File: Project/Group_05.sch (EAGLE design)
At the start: 29 parts, among them J1 POWER_JACKPTH_LOCK, U1 +12v, U3 TCA9546A_SMD

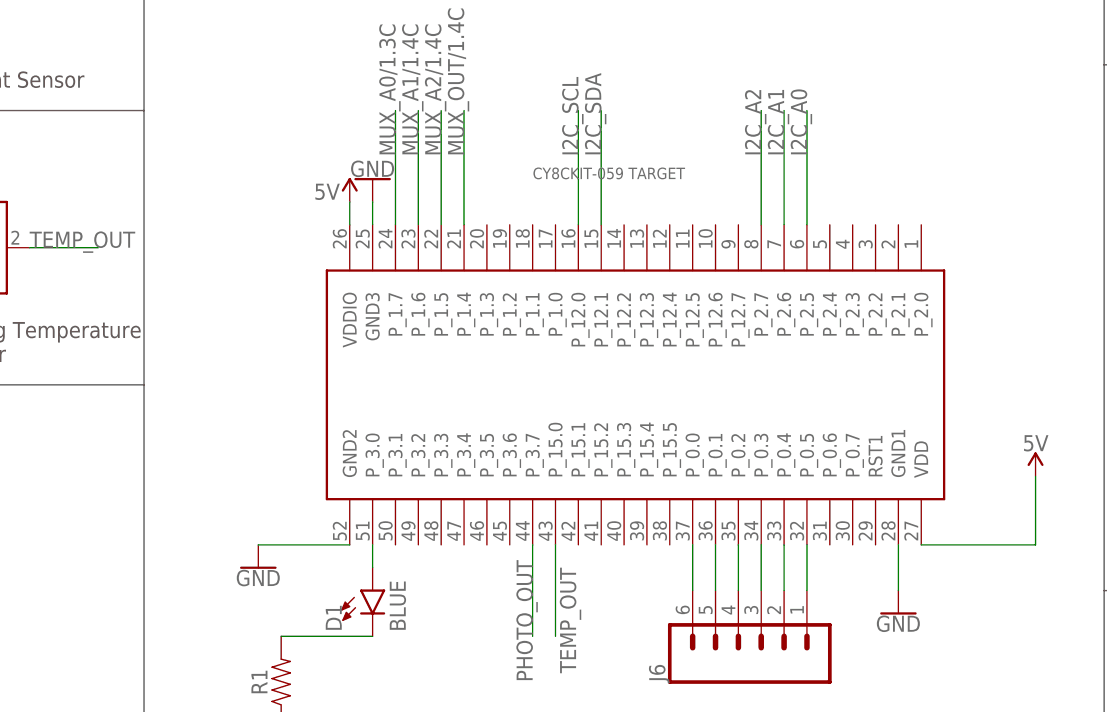
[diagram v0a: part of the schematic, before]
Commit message: brd placement
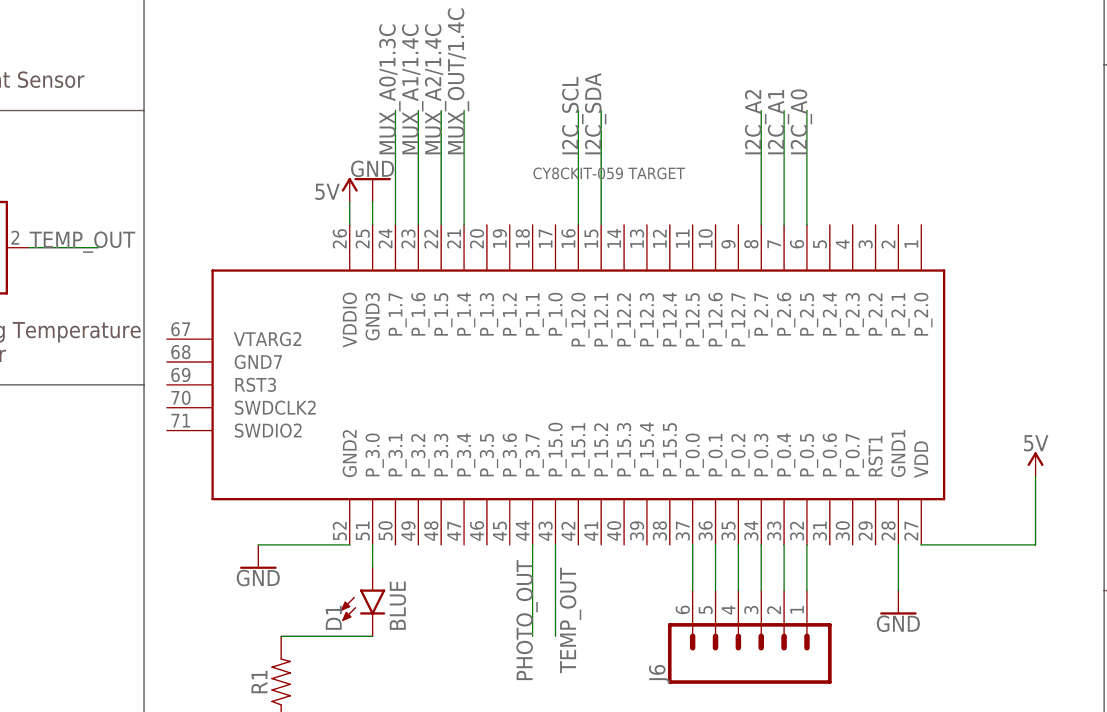
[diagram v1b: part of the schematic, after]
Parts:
- removed U$3: CY8CKIT-059_TARGET_3, CY8KIT-059:CY8CKIT-059_TARGET_3
- added U$1: CY8CKIT-059_TARGET, CY8KIT-059:CY8CKIT-059_TARGET
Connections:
- net 5V: now also U$1.VDD, U$1.VDDIO; no longer U$3.VDD, U$3.VDDIO
- net GND: now also U$1.GND1, U$1.GND2, U$1.GND3; no longer U$3.GND1, U$3.GND2, U$3.GND3
- net I2C_A0: now also U$1.P_2.5; no longer U$3.P_2.5
- net I2C_A1: now also U$1.P_2.6; no longer U$3.P_2.6
- net I2C_A2: now also U$1.P_2.7; no longer U$3.P_2.7
- net I2C_SCL: now also U$1.P_12.0; no longer U$3.P_12.0
- net I2C_SDA: now also U$1.P_12.1; no longer U$3.P_12.1
- net MUX_A0/1.3C: now also U$1.P_1.7; no longer U$3.P_1.7
- net MUX_A1/1.4C: now also U$1.P_1.6; no longer U$3.P_1.6
- net MUX_A2/1.4C: now also U$1.P_1.5; no longer U$3.P_1.5
- net MUX_OUT/1.4C: now also U$1.P_1.4; no longer U$3.P_1.4
- net N$1: now also U$1.P_0.0; no longer U$3.P_0.0
- net N$2: now also U$1.P_3.0; no longer U$3.P_3.0
- net N$5: now also U$1.P_0.1; no longer U$3.P_0.1
- net N$6: now also U$1.P_0.2; no longer U$3.P_0.2
- net N$7: now also U$1.P_0.3; no longer U$3.P_0.3
- net N$8: now also U$1.P_0.4; no longer U$3.P_0.4
- net N$9: now also U$1.P_0.5; no longer U$3.P_0.5
- net PHOTO_OUT: now also U$1.P_3.7; no longer U$3.P_3.7
- net TEMP_OUT: now also U$1.P_15.0; no longer U$3.P_15.0
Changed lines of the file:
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@@
 <part name="SUPPLY11" library="SparkFun-PowerSymbols" deviceset="5V" device=""/>
 <part name="U$2" library="Group_05_Library" deviceset="TMUX1208" device="_SMD"/>
-<part name="U$3" library="CY8KIT-059" deviceset="CY8CKIT-059_TARGET_3" device=""/>
 <part name="J8" library="SparkFun-Connectors" deviceset="CONN_08" device="LOCK"/>
 <part name="GND4" library="SparkFun-PowerSymbols" deviceset="GND" device=""/>
 <part name="GND5" library="SparkFun-PowerSymbols" deviceset="GND" device=""/>
 <part name="SUPPLY9" library="SparkFun-PowerSymbols" deviceset="5V" device=""/>
+<part name="U$1" library="CY8KIT-059" deviceset="CY8CKIT-059_TARGET" device=""/>
 </parts>
 <sheets>
@@
 <attribute name="VALUE" x="218.44" y="50.8" size="2.54" layer="96"/>
 </instance>
-<instance part="U$3" gate="G$1" x="93.98" y="71.12" smashed="yes"/>
 <instance part="J8" gate="G$1" x="187.96" y="55.88" smashed="yes">
 <attribute name="VALUE" x="182.88" y="43.434" size="1.778" layer="96" font="vector"/>
@@
 <attribute name="VALUE" x="60.96" y="91.694" size="1.778" layer="96" align="bottom-center"/>
 </instance>
+<instance part="U$1" gate="G$1" x="40.64" y="71.12" smashed="yes"/>
 </instances>
 <busses>
@@
 <pinref part="GND8" gate="1" pin="GND"/>
 <wire x1="124.46" y1="53.34" x2="124.46" y2="48.26" width="0.1524" layer="91"/>
-<pinref part="U$3" gate="G$1" pin="GND1"/>
+<pinref part="U$1" gate="G$1" pin="GND1"/>
 </segment>
 <segment>
@@
 <segment>
 <pinref part="GND4" gate="1" pin="GND"/>
-<pinref part="U$3" gate="G$1" pin="GND2"/>
 <wire x1="53.34" y1="53.34" x2="63.5" y2="53.34" width="0.1524" layer="91"/>
+<pinref part="U$1" gate="G$1" pin="GND2"/>
 </segment>
 <segment>
 <pinref part="GND5" gate="1" pin="GND"/>
-<pinref part="U$3" gate="G$1" pin="GND3"/>
 <wire x1="66.04" y1="91.44" x2="66.04" y2="88.9" width="0.1524" layer="91"/>
+<pinref part="U$1" gate="G$1" pin="GND3"/>
 </segment>
 </net>
@@
 <wire x1="139.7" y1="53.34" x2="139.7" y2="60.96" width="0.1524" layer="91"/>
 <pinref part="SUPPLY8" gate="G$1" pin="5V"/>
-<pinref part="U$3" gate="G$1" pin="VDD"/>
+<pinref part="U$1" gate="G$1" pin="VDD"/>
 </segment>
 <segment>
@@
 <segment>
 <pinref part="SUPPLY9" gate="G$1" pin="5V"/>
-<pinref part="U$3" gate="G$1" pin="VDDIO"/>
+<pinref part="U$1" gate="G$1" pin="VDDIO"/>
 <wire x1="63.5" y1="91.44" x2="63.5" y2="88.9" width="0.1524" layer="91"/>
 </segment>
@@
 <wire x1="83.82" y1="53.34" x2="83.82" y2="43.18" width="0.1524" layer="91"/>
 <label x="83.82" y="38.1" size="1.778" layer="95" rot="R90"/>
-<pinref part="U$3" gate="G$1" pin="P_3.7"/>
+<pinref part="U$1" gate="G$1" pin="P_3.7"/>
 </segment>
 </net>
@@
 <wire x1="86.36" y1="53.34" x2="86.36" y2="43.18" width="0.1524" layer="91"/>
 <label x="86.868" y="50.8" size="1.778" layer="95" rot="R270"/>
-<pinref part="U$3" gate="G$1" pin="P_15.0"/>
+<pinref part="U$1" gate="G$1" pin="P_15.0"/>
 </segment>
 </net>
@@
 <wire x1="91.44" y1="88.9" x2="91.44" y2="101.6" width="0.1524" layer="91"/>
 <label x="91.44" y="96.52" size="1.778" layer="95" rot="R90"/>
-<pinref part="U$3" gate="G$1" pin="P_12.1"/>
+<pinref part="U$1" gate="G$1" pin="P_12.1"/>
 </segment>
 </net>
@@
 <wire x1="88.9" y1="88.9" x2="88.9" y2="101.6" width="0.1524" layer="91"/>
 <label x="88.9" y="96.52" size="1.778" layer="95" rot="R90"/>
-<pinref part="U$3" gate="G$1" pin="P_12.0"/>
+<pinref part="U$1" gate="G$1" pin="P_12.0"/>
 </segment>
 </net>
@@
 <wire x1="114.3" y1="88.9" x2="114.3" y2="101.6" width="0.1524" layer="91"/>
 <label x="114.3" y="96.52" size="1.778" layer="95" rot="R90"/>
-<pinref part="U$3" gate="G$1" pin="P_2.5"/>
+<pinref part="U$1" gate="G$1" pin="P_2.5"/>
 </segment>
 </net>
@@
 <wire x1="111.76" y1="88.9" x2="111.76" y2="101.6" width="0.1524" layer="91"/>
 <label x="111.76" y="96.52" size="1.778" layer="95" rot="R90"/>
-<pinref part="U$3" gate="G$1" pin="P_2.6"/>
+<pinref part="U$1" gate="G$1" pin="P_2.6"/>
 </segment>
 </net>
@@
 <wire x1="109.22" y1="88.9" x2="109.22" y2="101.6" width="0.1524" layer="91"/>
 <label x="109.22" y="96.52" size="1.778" layer="95" rot="R90"/>
-<pinref part="U$3" gate="G$1" pin="P_2.7"/>
+<pinref part="U$1" gate="G$1" pin="P_2.7"/>
 </segment>
 </net>
@@
 <pinref part="D1" gate="G$1" pin="A"/>
 <wire x1="66.04" y1="53.34" x2="66.04" y2="50.8" width="0.1524" layer="91"/>
-<pinref part="U$3" gate="G$1" pin="P_3.0"/>
+<pinref part="U$1" gate="G$1" pin="P_3.0"/>
 </segment>
 </net>
@@
 <pinref part="J6" gate="G$1" pin="6"/>
 <wire x1="101.6" y1="53.34" x2="101.6" y2="48.26" width="0.1524" layer="91"/>
-<pinref part="U$3" gate="G$1" pin="P_0.0"/>
+<pinref part="U$1" gate="G$1" pin="P_0.0"/>
 </segment>
 </net>
@@
 <pinref part="J6" gate="G$1" pin="5"/>
 <wire x1="104.14" y1="53.34" x2="104.14" y2="48.26" width="0.1524" layer="91"/>
-<pinref part="U$3" gate="G$1" pin="P_0.1"/>
+<pinref part="U$1" gate="G$1" pin="P_0.1"/>
 </segment>
 </net>
@@
 <pinref part="J6" gate="G$1" pin="4"/>
 <wire x1="106.68" y1="53.34" x2="106.68" y2="48.26" width="0.1524" layer="91"/>
-<pinref part="U$3" gate="G$1" pin="P_0.2"/>
+<pinref part="U$1" gate="G$1" pin="P_0.2"/>
 </segment>
 </net>
@@
 <pinref part="J6" gate="G$1" pin="3"/>
 <wire x1="109.22" y1="53.34" x2="109.22" y2="48.26" width="0.1524" layer="91"/>
-<pinref part="U$3" gate="G$1" pin="P_0.3"/>
+<pinref part="U$1" gate="G$1" pin="P_0.3"/>
 </segment>
 </net>
@@
 <pinref part="J6" gate="G$1" pin="2"/>
 <wire x1="111.76" y1="53.34" x2="111.76" y2="48.26" width="0.1524" layer="91"/>
-<pinref part="U$3" gate="G$1" pin="P_0.4"/>
+<pinref part="U$1" gate="G$1" pin="P_0.4"/>
 </segment>
 </net>
@@
 <pinref part="J6" gate="G$1" pin="1"/>
 <wire x1="114.3" y1="53.34" x2="114.3" y2="48.26" width="0.1524" layer="91"/>
-<pinref part="U$3" gate="G$1" pin="P_0.5"/>
+<pinref part="U$1" gate="G$1" pin="P_0.5"/>
 </segment>
 </net>
@@
 <wire x1="68.58" y1="88.9" x2="68.58" y2="101.6" width="0.1524" layer="91"/>
 <label x="68.58" y="96.52" size="1.778" layer="95" rot="R90"/>
-<pinref part="U$3" gate="G$1" pin="P_1.7"/>
+<pinref part="U$1" gate="G$1" pin="P_1.7"/>
 </segment>
 </net>
@@
 <wire x1="71.12" y1="88.9" x2="71.12" y2="101.6" width="0.1524" layer="91"/>
 <label x="71.12" y="96.52" size="1.778" layer="95" rot="R90"/>
-<pinref part="U$3" gate="G$1" pin="P_1.6"/>
+<pinref part="U$1" gate="G$1" pin="P_1.6"/>
 </segment>
 </net>
@@
 <wire x1="73.66" y1="88.9" x2="73.66" y2="101.6" width="0.1524" layer="91"/>
 <label x="73.66" y="96.52" size="1.778" layer="95" rot="R90"/>
-<pinref part="U$3" gate="G$1" pin="P_1.5"/>
+<pinref part="U$1" gate="G$1" pin="P_1.5"/>
 </segment>
 </net>
@@
 <wire x1="76.2" y1="88.9" x2="76.2" y2="101.6" width="0.1524" layer="91"/>
 <label x="76.2" y="96.52" size="1.778" layer="95" rot="R90"/>
-<pinref part="U$3" gate="G$1" pin="P_1.4"/>
-</segment>
-</net>
+<pinref part="U$1" gate="G$1" pin="P_1.4"/>
+</segment>
+</net>
